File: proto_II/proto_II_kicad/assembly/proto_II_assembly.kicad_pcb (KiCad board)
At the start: 2 copper layers, 100 x 97 mm, 107 parts, among them J1 BOOT_CFG, J2 SNSR_I2C, J3 SNSR_PWR, J4 Vin, J5 RS485_A, J6 RS485_B, J7 ISO_GND, J8 SWD_DBG, SW1 RST, SW2 MODBUS_ADDR, SW3 USR_BTN, U1 STM32F103C8Tx, U2 TPS54331, U3 XC6206P332MR, U4 ADM2587E, Y1 HSE, Y2 LSE

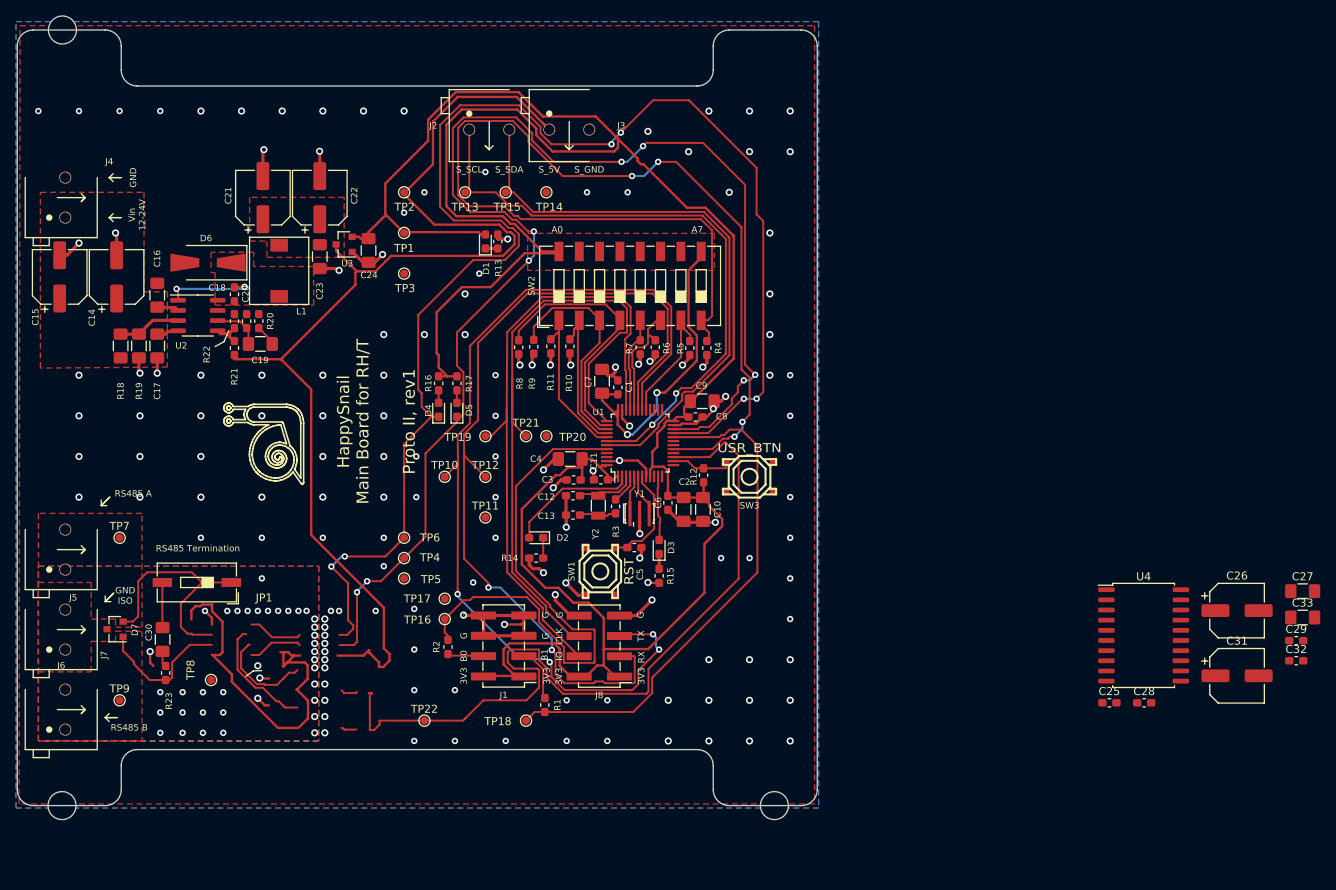
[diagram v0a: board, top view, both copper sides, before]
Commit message: tmp: more work
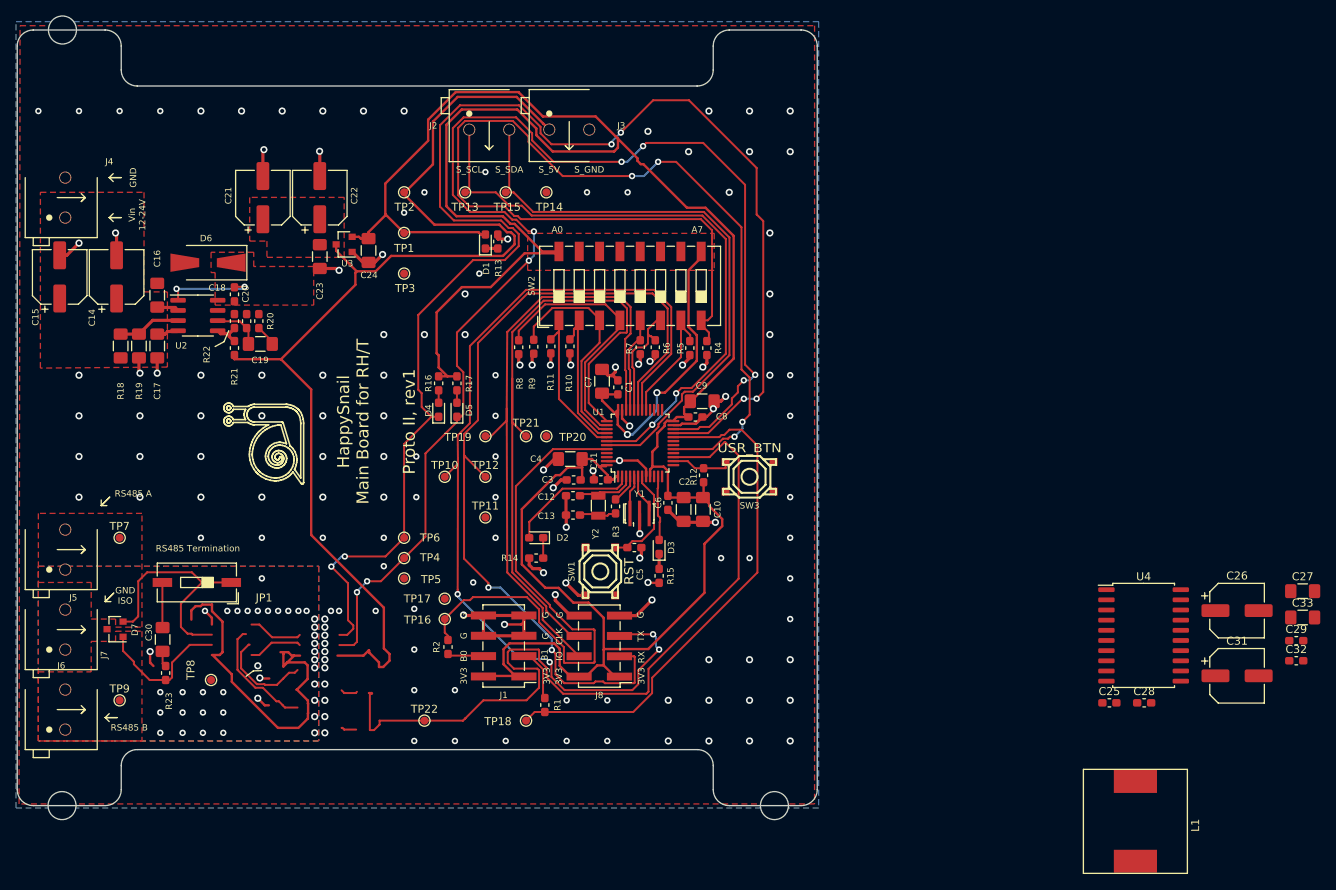
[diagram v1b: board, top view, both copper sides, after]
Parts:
- L1: value 22u -> 47u; footprint Project:CDRH74 -> Project:SWRB1205S
- moved L1 127.2 mm to (177.8, 132.0), turned to 270 degrees
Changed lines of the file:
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@@
     (uvia_drill 0.1)
   )
+  (module Project:SWRB1205S (layer F.Cu)
+    (at 177.77206 131.96952 270)
+    (descr "Sunlord Wire Wound SMD Power Inductors – SWRB-S Series")
+    (tags Sunlord,SWRB1205S,Inductor,choke,coil)
+    (attr smd)
+    (fp_text reference L1 (at 0.5 -7.5 90) (layer F.SilkS)
+      (effects (font (size 1 1) (thickness 0.15)))
+    )
+    (fp_text value 47u (at 0 -9 90) (layer F.Fab)
+      (effects (font (size 1 1) (thickness 0.15)))
+    )
+    (fp_line (start -6.5 6.5) (end -6.5 -6.5) (layer F.SilkS) (width 0.15))
+    (fp_line (start 6.5 6.5) (end -6.5 6.5) (layer F.SilkS) (width 0.15))
+    (fp_line (start 6.5 -6.5) (end 6.5 6.5) (layer F.SilkS) (width 0.15))
+    (fp_line (start -6.5 -6.5) (end 6.5 -6.5) (layer F.SilkS) (width 0.15))
+    (fp_line (start -6.5 -6.5) (end 0 -6.5) (layer F.CrtYd) (width 0.02))
+    (fp_line (start -6.5 0) (end -6.5 -6.5) (layer F.CrtYd) (width 0.02))
+    (fp_line (start -6.5 6.5) (end -6.5 0) (layer F.CrtYd) (width 0.02))
+    (fp_line (start 0 6.5) (end -6.5 6.5) (layer F.CrtYd) (width 0.02))
+    (fp_line (start 6.5 6.5) (end 0 6.5) (layer F.CrtYd) (width 0.02))
+    (fp_line (start 6.5 0) (end 6.5 6.5) (layer F.CrtYd) (width 0.02))
+    (fp_line (start 6.5 -6.5) (end 6.5 0) (layer F.CrtYd) (width 0.02))
+    (fp_line (start 0 -6.5) (end 6.5 -6.5) (layer F.CrtYd) (width 0.02))
+    (pad 2 smd rect (at 5 0 270) (size 2.9 5.4) (layers F.Cu F.Paste F.Mask)
+      (net 6 +5V))
+    (pad 1 smd rect (at -5 0 270) (size 2.9 5.4) (layers F.Cu F.Paste F.Mask)
+      (net 5 /power/PH))
+    (model ${KIPRJMOD}/../common/3d/CDRN74.stp
+      (at (xyz 0 0 0))
+      (scale (xyz 1 1 1))
+      (rotate (xyz -90 0 0))
+    )
+  )
   (module Package_SO:SOIC-20W_7.5x12.8mm_P1.27mm (layer F.Cu)
     (at 178.79832 108.72496)
@@
     )
   )
-  (module Project:CDRH74 (layer F.Cu)
-    (at 70.7395 63.1515 180)
-    (descr "Sumidia SMD Power Inductor ")
-    (tags Sumidia,CDRH74,Inductor,choke,coil)
-    (attr smd)
-    (fp_text reference L1 (at -2.794 -5.08) (layer F.SilkS)
-      (effects (font (size 0.8 0.8) (thickness 0.15)))
-    )
-    (fp_text value 22u (at 0 -6.5) (layer F.Fab)
-      (effects (font (size 1 1) (thickness 0.15)))
-    )
-    (fp_line (start 3.7 -4.2) (end 3.7 4.2) (layer F.SilkS) (width 0.15))
-    (fp_line (start -3.7 4.2) (end -3.7 -4.2) (layer F.SilkS) (width 0.15))
-    (fp_line (start -3.7 -4.2) (end 3.7 -4.2) (layer F.SilkS) (width 0.15))
-    (fp_line (start 3.7 4.2) (end -3.7 4.2) (layer F.SilkS) (width 0.15))
-    (fp_line (start -3.7 -4.2) (end 3.7 -4.2) (layer F.CrtYd) (width 0.02))
-    (fp_line (start 3.7 -4.2) (end 3.7 4.2) (layer F.CrtYd) (width 0.02))
-    (fp_line (start 3.7 4.2) (end -3.7 4.2) (layer F.CrtYd) (width 0.02))
-    (fp_line (start -3.7 4.2) (end -3.7 -4.2) (layer F.CrtYd) (width 0.02))
-    (pad 1 smd rect (at 0 -3.2 180) (size 2.2 1.6) (layers F.Cu F.Paste F.Mask)
-      (net 5 /power/PH))
-    (pad 2 smd rect (at 0 3.2 180) (size 2.2 1.6) (layers F.Cu F.Paste F.Mask)
-      (net 6 +5V))
-    (model ${KIPRJMOD}/../common/3d/CDRN74.stp
-      (at (xyz 0 0 0))
-      (scale (xyz 1 1 1))
-      (rotate (xyz -90 0 0))
-    )
-  )
